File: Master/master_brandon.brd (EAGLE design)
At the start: 76.8 x 60.3 mm, 58 parts, among them J1 ISP, K1 653002114822, K2 653002114822, K3 653002114822, K4 653002114822, U1 ATMEGA128RFA1, U3 ULN2003ANE4, Y1 16MHz, Y2 32.768kHz

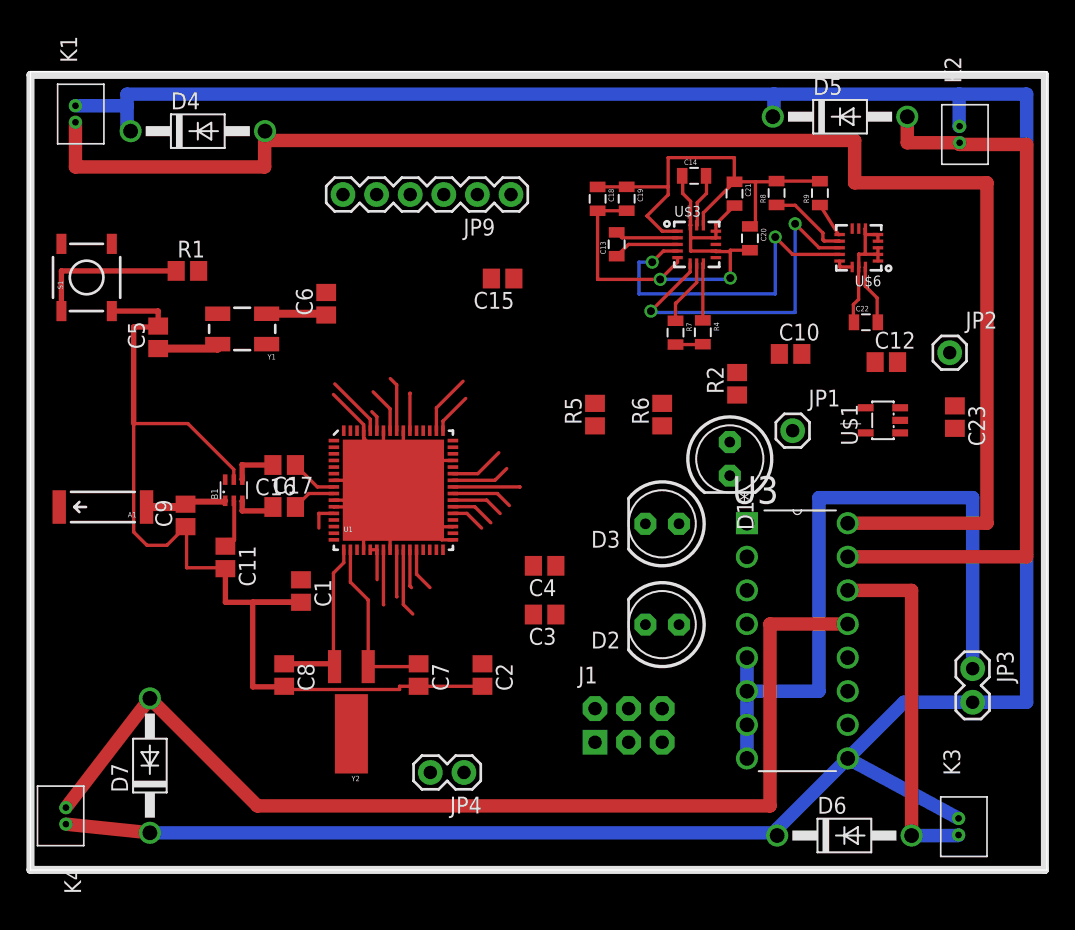
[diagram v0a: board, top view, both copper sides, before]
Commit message: updated Brandon's Master
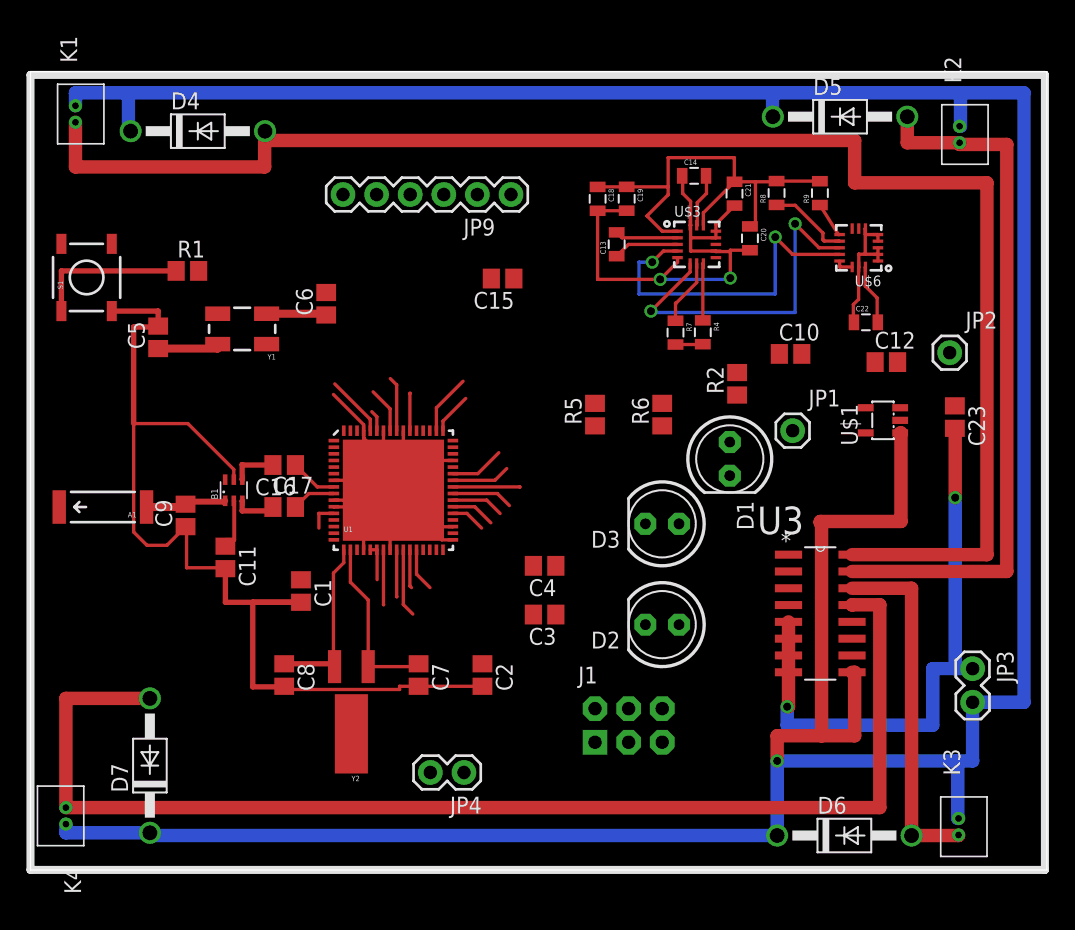
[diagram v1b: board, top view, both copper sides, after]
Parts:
- U3: value ULN2003ANE4 -> ULN2003ADR; device Texas Instruments_By_element14_Batch_1:DIP254P762X508-16 -> Texas Instruments_By_element14_Batch_1:SOIC127P600X175-16N
- moved U3 6.52 mm to (62.1, 12.4)
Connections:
- removed net VDD: C10.1, JP1.1, R2.2, U$1.5
- net 3.3V: now also C10.1, JP1.1, R2.2, U$1.5
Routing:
- net VCC: track 211.8 -> 255.9 mm, vias 0 -> 1
- net N$26: track 80.3 -> 93.6 mm
- net GND: track 225.9 -> 218.0 mm, vias 2 -> 4
- net N$24: track 55.8 -> 53.6 mm
- net N$29: track 115.1 -> 117.2 mm
